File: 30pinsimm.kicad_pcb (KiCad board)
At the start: 4 copper layers, 89 x 16.6 mm, 7 parts, among them U1 JEDEC-FPDRAM_xMbx4, U2 JEDEC-FPDRAM_xMbx4, U3 JEDEC-FPDRAM_xMbx1

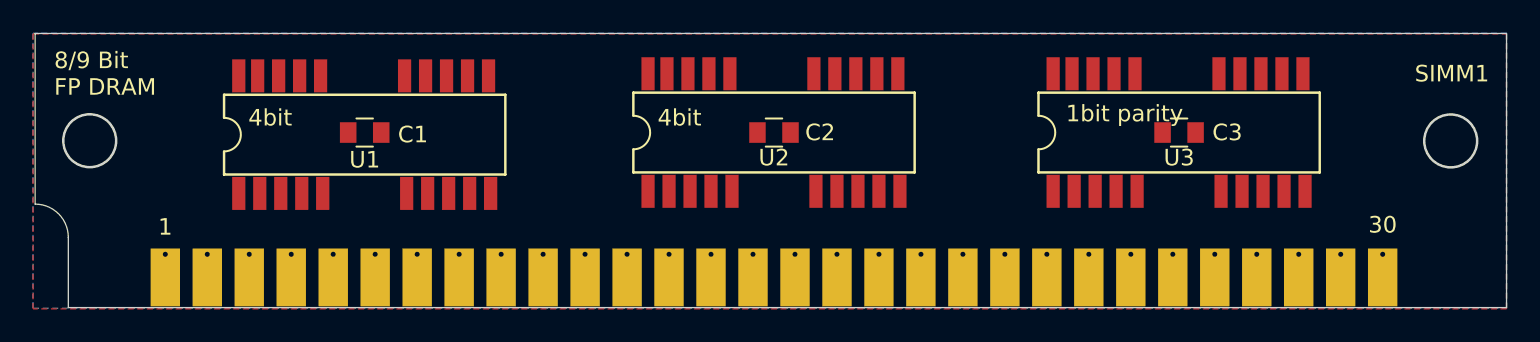
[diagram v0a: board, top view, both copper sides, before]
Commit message: alingment
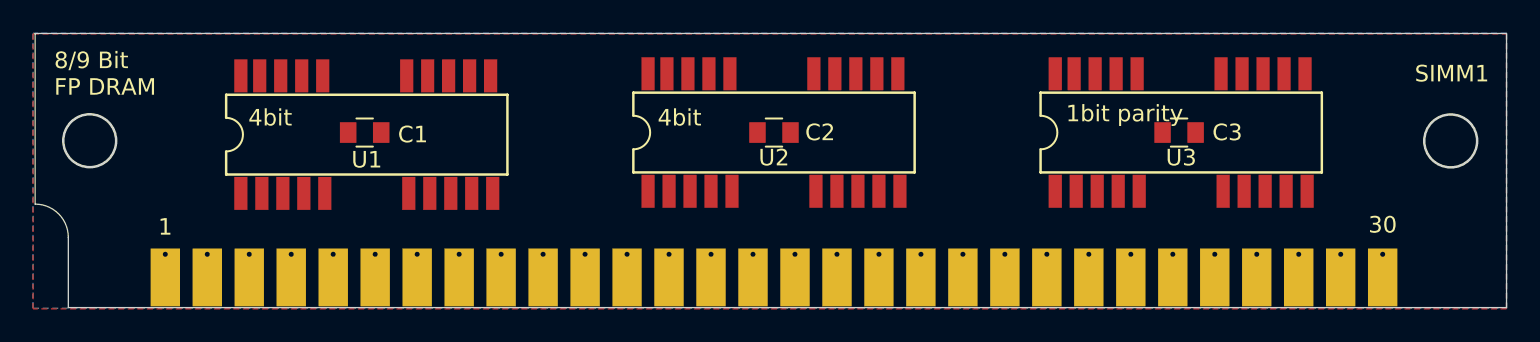
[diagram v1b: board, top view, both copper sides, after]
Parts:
- moved U1 0.13 mm to (119.5, 100.8)
- moved U3 0.13 mm to (168.8, 100.7)
